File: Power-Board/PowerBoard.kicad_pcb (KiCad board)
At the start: 2 copper layers, 76.2 x 102.9 mm, 59 parts, among them J1 IN1, J10 probe3, J11 Battery_out, J12 Buck_out, J13 IN2, J14 Boost_out, J15 Buck_out, J16 Conn_01x02_Male, J17 Conn_01x02_Male, J2 Conn_02x13_Odd_Even, J3 Boost, J4 Buck, J5 Buck_out, J6 probe1, J7 probe4, J8 bmp388, J9 probe2, Q1 SIS427EDN-T1-GE3, Q2 MMBT3906, Q3 SIS427EDN-T1-GE3, U1 Pico, U2 BMP388, U3 TMUX1104DGSR, U4 LM7805_TO220

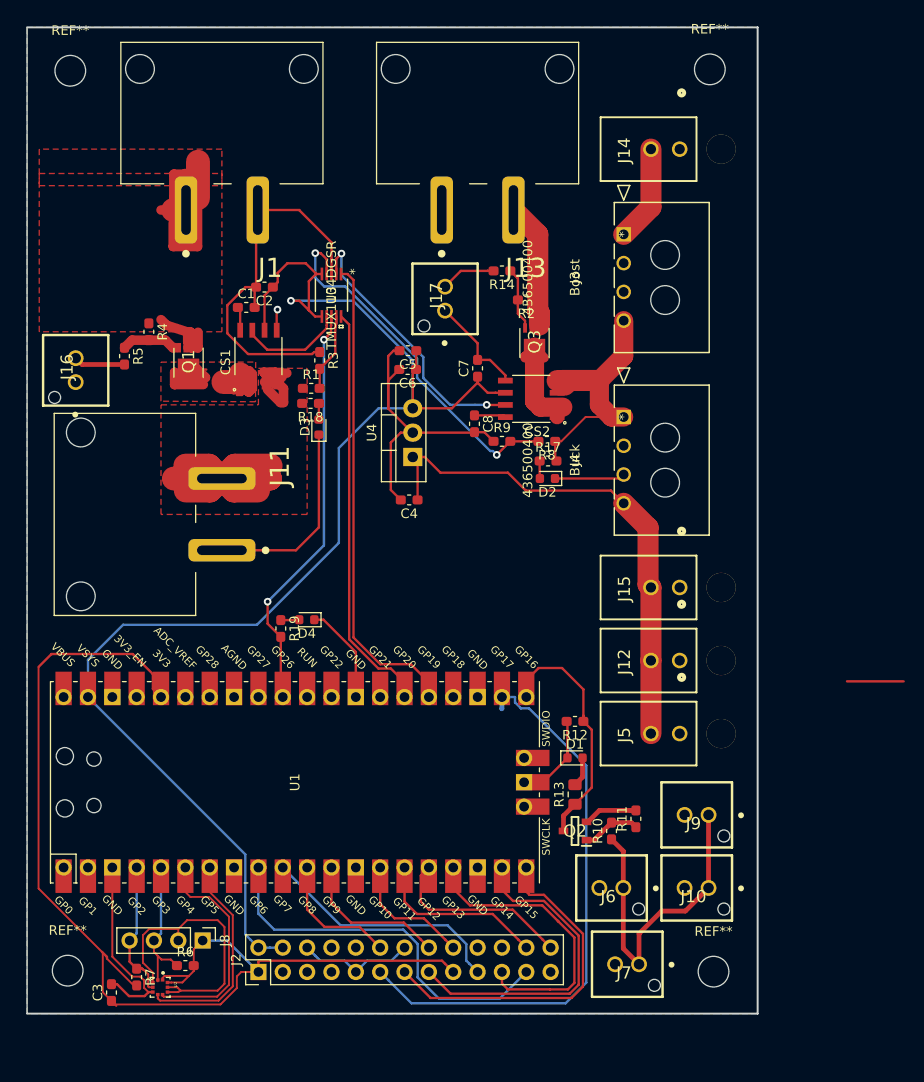
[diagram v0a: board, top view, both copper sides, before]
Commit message: Power Board completed
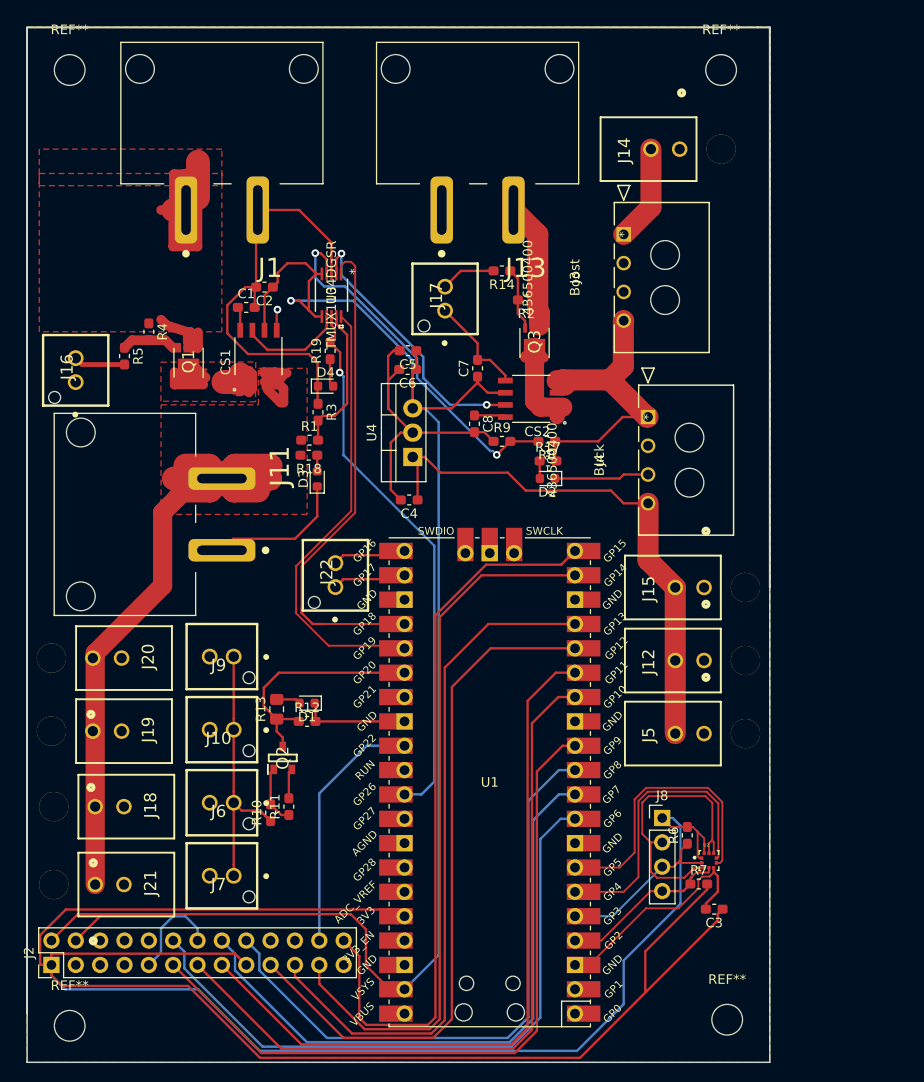
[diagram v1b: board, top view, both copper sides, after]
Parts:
- removed the REF** at (80.4, 145.4)
- removed the REF** at (147.8, 145.5)
- removed the REF** at (147.4, 51.4)
- removed the REF** at (80.7, 51.5)
- added J18: Battery_out, footprint:input, F.Cu at (79.0, 128.3)
- added J19: Battery_out, footprint:input, F.Cu at (78.7, 120.4)
- added J20: Battery_out, footprint:input, F.Cu at (78.7, 112.8)
- added J21: Battery_out, footprint:input, F.Cu at (79.0, 136.4)
- added J22: Conn_01x02_Male, footprint:01x02, F.Cu at (111.8, 104.1)
- added REF**: MountingHole_3.2mm_M3, MountingHole:MountingHole_3.2mm_M3, F.Cu at (80.6, 151.1)
- added REF**: MountingHole_3.2mm_M3, MountingHole:MountingHole_3.2mm_M3, F.Cu at (149.2, 150.5)
- added REF**: MountingHole_3.2mm_M3, MountingHole:MountingHole_3.2mm_M3, F.Cu at (148.6, 51.4)
- added REF**: MountingHole_3.2mm_M3, MountingHole:MountingHole_3.2mm_M3, F.Cu at (80.6, 51.4)
- moved C3 63.5 mm to (147.9, 139.0), turned to 180 degrees
- moved R7 59.4 mm to (146.3, 136.3), turned to 0 degrees
- moved U2 58.8 mm to (147.3, 133.9), turned to 0 degrees
- moved R6 54.1 mm to (145.1, 131.3), turned to 90 degrees
- moved J9 52.2 mm to (96.5, 109.2)
- moved J10 52.2 mm to (96.5, 116.8)
- moved J8 49.6 mm to (142.4, 129.5), turned to 0 degrees
- moved J7 43.3 mm to (96.5, 132.1)
- moved J6 41.6 mm to (96.5, 124.5)
- moved R11 36.2 mm to (103.5, 128.3)
- moved R10 35.6 mm to (101.6, 128.9)
- moved R13 32.4 mm to (102.2, 118.1)
- moved Q2 31.4 mm to (102.9, 123.2), turned to 90 degrees
- moved R19 29.4 mm to (107.8, 80.7), turned to 90 degrees
- moved D1 28.5 mm to (105.4, 117.5), turned to 180 degrees
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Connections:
- U1 pad 10: /SI -> /K2
- U1 pad 11: /K1 -> /K3
- U1 pad 12: /K2 -> /TP_IRQ
- U1 pad 14: /K3 -> /RST
- U1 pad 15: /LCD_CS -> /RS
- U1 pad 16: /TP_CS -> /SI
- U1 pad 19: /RS -> /SCK
- U1 pad 20: /RST -> /TP_CS
- U1 pad 21: /leak_signal -> /TX
- U1 pad 22: /TP_IRQ -> /RX
- U1 pad 24: Net-(U1-Pad24) -> /CTRL1
- U1 pad 25: /CTRL1 -> /CTRL2
- U1 pad 26: /CTRL2 -> /leak_signal
- U1 pad 29: Net-(U1-Pad29) -> /LCD_CS
- U1 pad 9: /SCK -> /K1
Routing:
- net /3.3V: track 116.5 -> 261.9 mm
- net /TP_CS: track 19.4 -> 76.6 mm
- net /K1: track 13.6 -> 68.3 mm
- net /K3: track 13.3 -> 64.3 mm
- net /K2: track 15.8 -> 65.1 mm
- net /RV1: track 41.4 -> 90.0 mm
- net /SI: track 25.9 -> 72.0 mm
- net /RS: track 34.4 -> 76.3 mm
- net /RST: track 36.0 -> 76.9 mm
- net /TP_SO: track 31.2 -> 72.1 mm
- net /SCK: track 39.6 -> 74.8 mm
- net /5V: track 148.8 -> 169.6 mm
- net /TP_IRQ: track 59.7 -> 74.8 mm
- net /MOUT: track 43.1 -> 57.1 mm, vias 2 -> 1
- net /LCD_CS: track 18.2 -> 26.3 mm
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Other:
- board size 76.2 x 102.9 mm -> 77.5 x 107.9 mm

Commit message: issue resolved
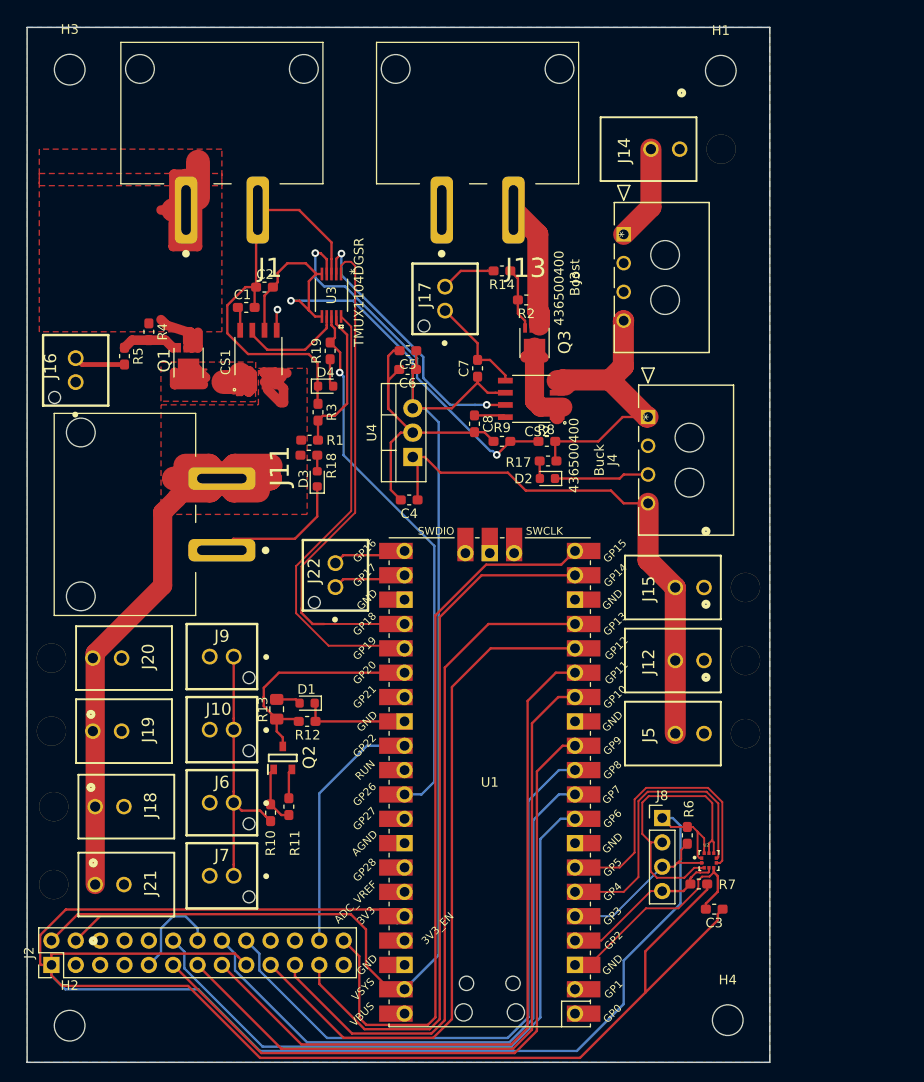
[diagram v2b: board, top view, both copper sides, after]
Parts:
- removed REF** (x4): MountingHole_3.2mm_M3, MountingHole:MountingHole_3.2mm_M3
- added H1: MountingHole, MountingHole:MountingHole_3.2mm_M3, F.Cu at (148.6, 51.5)
- added H2: MountingHole, MountingHole:MountingHole_3.2mm_M3, F.Cu at (80.6, 151.1)
- added H3: MountingHole, MountingHole:MountingHole_3.2mm_M3, F.Cu at (80.6, 51.4)
- added H4: MountingHole, MountingHole:MountingHole_3.2mm_M3, F.Cu at (149.3, 150.5)
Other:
- outline, holes or cut-outs redrawn
